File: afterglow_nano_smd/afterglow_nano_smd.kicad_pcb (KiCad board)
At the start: 2 copper layers, 113.7 x 80 mm, 112 parts, among them J1 J137_IN_C, J2 J133_IN_R, J3 Conn_Power, J4 J133_OUT_R, J5 J137_OUT_C, J6 J134_OUT_R, J7 J138_OUT_C, J8 J135_OUT_R, J9 136_OUT_C, Q1 IRF5305, Q10 IRL2905, Q11 IRL2905, Q12 IRL2905, Q13 IRL2905, Q14 IRL2905, Q15 IRL2905, Q16 IRL2905, Q2 IRF5305, Q3 IRF5305, Q4 IRF5305, Q5 IRF5305, Q6 IRF5305, Q7 IRF5305, Q8 IRF5305, Q9 IRL2905, SW1 CFG, U1 74LS165, U2 74LS165, U3 5V_Regulator, U4 arduino_nano, U5 74HC595, U6 74HC595, U7 ULN2803A

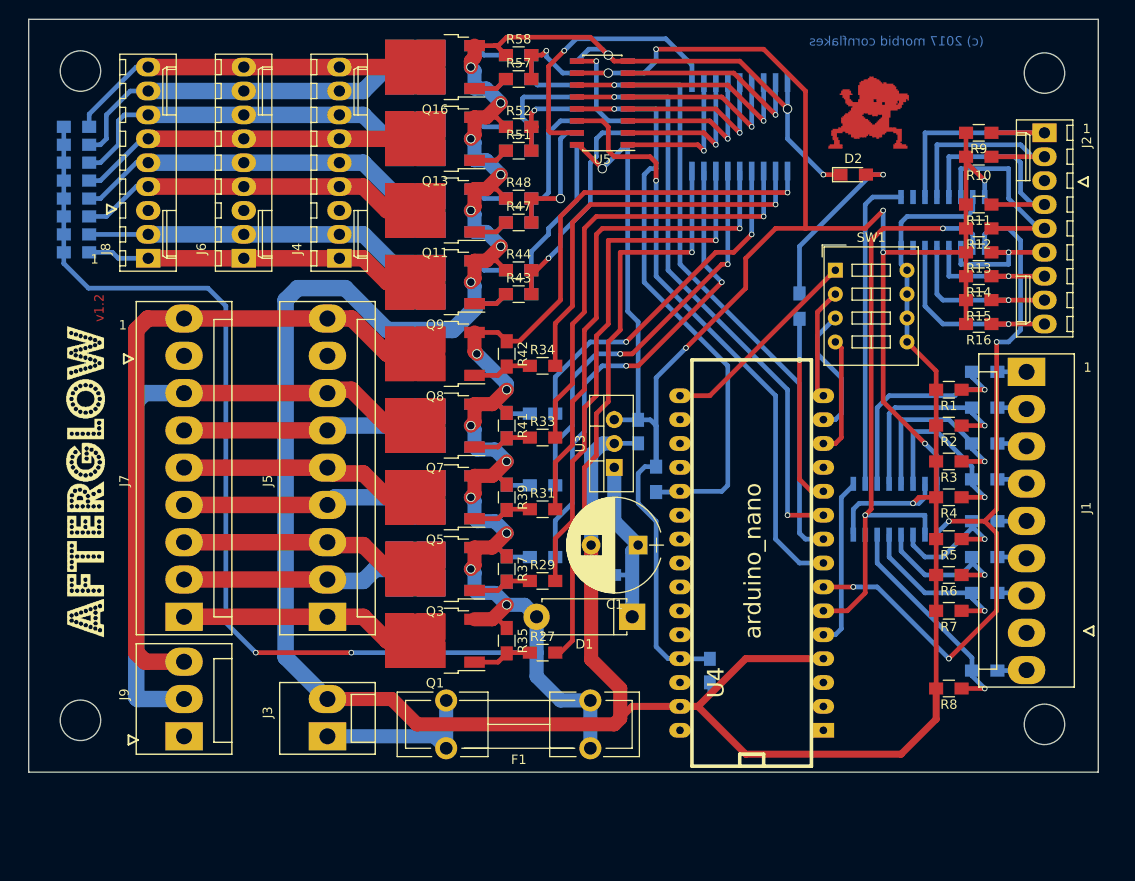
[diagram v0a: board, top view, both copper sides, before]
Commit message: v1.3 PCB progress
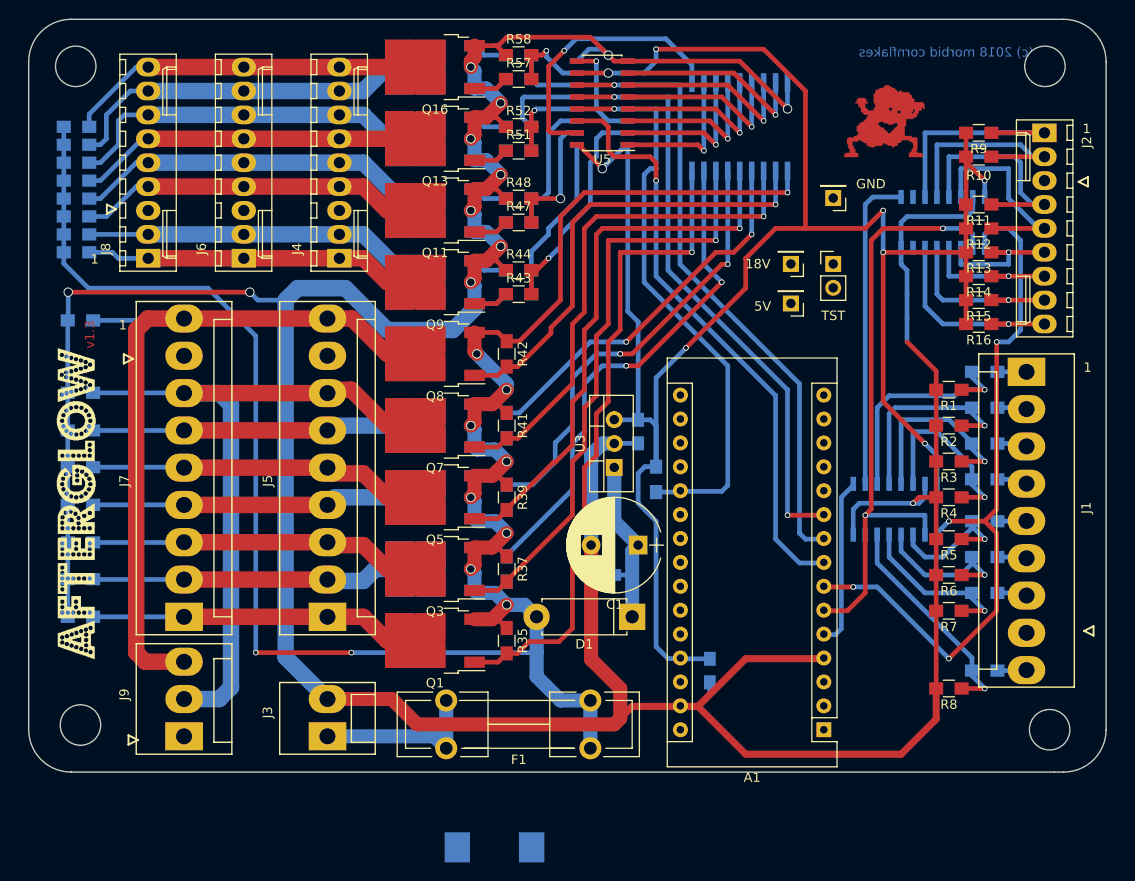
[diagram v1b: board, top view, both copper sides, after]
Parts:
- removed the ? at (132.9, 55.7)
- removed the ? at (30.5, 55.5)
- removed the ? at (30.5, 124.5)
- removed the ? at (132.9, 124.9)
- removed D2: LED, LEDs:LED_0805_HandSoldering
- removed SW1: CFG, Buttons_Switches_THT:SW_DIP_x4_W7.62mm_Slide
- removed U4: arduino_nano, arduino_nano:arduino_mini
- added 18V: TestPoint, Pin_Headers:Pin_Header_Straight_1x01_Pitch2.54mm, F.Cu at (106.0, 76.0)
- added 5V: TestPoint, Pin_Headers:Pin_Header_Straight_1x01_Pitch2.54mm, F.Cu at (106.0, 80.2)
- added ?: MountingHole_4.3mm_M4_ISO14580, Mounting_Holes:MountingHole_4.3mm_M4_ISO14580, F.Cu at (133.5, 125.5)
- added ?: MountingHole_4.3mm_M4_ISO14580, Mounting_Holes:MountingHole_4.3mm_M4_ISO14580, F.Cu at (133.0, 55.0)
- added ?: MountingHole_4.3mm_M4_ISO14580, Mounting_Holes:MountingHole_4.3mm_M4_ISO14580, F.Cu at (30.5, 125.0)
- added ?: MountingHole_4.3mm_M4_ISO14580, Mounting_Holes:MountingHole_4.3mm_M4_ISO14580, F.Cu at (30.0, 55.0)
- added A1: Arduino_Nano_v3.x, Modules:Arduino_Nano, F.Cu at (109.5, 125.5)
- added GND: TestPoint, Pin_Headers:Pin_Header_Straight_1x01_Pitch2.54mm, F.Cu at (110.5, 69.0)
- added TST: Jumper, Pin_Headers:Pin_Header_Straight_1x02_Pitch2.54mm, F.Cu at (110.5, 76.0)
- J1, J5, J7: footprint afterglow:Molex_KK-41791-9_9x3.96mm_Straight -> Connectors_Molex:Molex_KK-41791-9_9x3.96mm_Straight
- R1, R2, R3, R4, R5, R6, R7, R8: value 390 -> 330
- R26: value 220 -> 0.22; footprint Resistors_SMD:R_0805_HandSoldering -> Resistors_SMD:R_2512_HandSoldering
- R27, R29, R31, R33, R34: value 560 -> 10k; moved to B.Cu
- R28, R30, R32: value 560 -> 10k
- moved R26 66.0 mm to (74.5, 138.0), turned to 0 degrees
- moved R34 49.3 mm to (30.5, 82.0)
- moved R33 49.3 mm to (30.5, 89.7)
- moved R31 49.3 mm to (30.5, 97.6)
- moved R29 49.3 mm to (30.5, 105.6)
- moved R27 49.3 mm to (30.5, 113.5)
- moved R28 49.2 mm to (30.5, 109.5)
- moved R30 49.2 mm to (30.5, 101.6)
- moved R32 49.1 mm to (30.5, 93.7)
- moved afterglow 2.54 mm to (28.0, 118.0)
- moved FLAKIE 1.89 mm to (111.5, 57.0)
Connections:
- net VCC renamed /5V
- J1 pad 8: (no net) -> Net-(J1-Pad8)
- J2 pad 3: (no net) -> Net-(J2-Pad3)
- J4 pad 3: (no net) -> Net-(J4-Pad3)
- J5 pad 8: (no net) -> Net-(J5-Pad8)
- J6 pad 3: (no net) -> Net-(J6-Pad3)
- J7 pad 8: (no net) -> Net-(J7-Pad8)
- J8 pad 3: (no net) -> Net-(J8-Pad3)
- J9 pad 1: (no net) -> Net-(J9-Pad1)
- Q1 pad 1: Net-(Q1-Pad1) -> /CO1
- Q10 pad 3: GND -> /ROW_GND
- Q11 pad 3: GND -> /ROW_GND
- Q12 pad 3: GND -> /ROW_GND
- Q13 pad 3: GND -> /ROW_GND
- Q14 pad 3: GND -> /ROW_GND
- Q15 pad 3: GND -> /ROW_GND
- Q16 pad 3: GND -> /ROW_GND
- Q2 pad 1: Net-(Q2-Pad1) -> /CO2
- Q3 pad 1: Net-(Q3-Pad1) -> /CO3
- Q4 pad 1: Net-(Q4-Pad1) -> /CO4
- Q5 pad 1: Net-(Q5-Pad1) -> /CO5
- Q6 pad 1: Net-(Q6-Pad1) -> /CO6
- Q7 pad 1: Net-(Q7-Pad1) -> /CO7
- Q8 pad 1: Net-(Q8-Pad1) -> /CO8
- Q9 pad 3: GND -> /ROW_GND
- R26 pad 1: Net-(D2-Pad2) -> GND
- R26 pad 2: Net-(R26-Pad2) -> /ROW_GND
- R27 pad 1: Net-(Q1-Pad1) -> GND
- R27 pad 2: /CO1 -> /J137_CO1
- R28 pad 1: Net-(Q2-Pad1) -> GND
- R28 pad 2: /CO2 -> /J137_CO2
- R29 pad 1: Net-(Q3-Pad1) -> GND
- R29 pad 2: /CO3 -> /J137_CO3
- R30 pad 1: Net-(Q4-Pad1) -> GND
- R30 pad 2: /CO4 -> /J137_CO4
- R31 pad 1: Net-(Q5-Pad1) -> GND
- R31 pad 2: /CO5 -> /J137_CO5
- R32 pad 1: Net-(Q6-Pad1) -> GND
- R32 pad 2: /CO6 -> /J137_CO6
- R33 pad 1: Net-(Q7-Pad1) -> GND
- R33 pad 2: /CO7 -> /J137_CO7
- R34 pad 1: Net-(Q8-Pad1) -> GND
- R34 pad 2: /CO8 -> /J137_CO8
- R35 pad 2: Net-(Q1-Pad1) -> /CO1
- R36 pad 2: Net-(Q2-Pad1) -> /CO2
- R37 pad 2: Net-(Q3-Pad1) -> /CO3
- R38 pad 2: Net-(Q4-Pad1) -> /CO4
- R39 pad 2: Net-(Q5-Pad1) -> /CO5
- R40 pad 2: Net-(Q6-Pad1) -> /CO6
- R41 pad 2: Net-(Q7-Pad1) -> /CO7
- R42 pad 2: Net-(Q8-Pad1) -> /CO8
- R44 pad 1: GND -> /ROW_GND
- R46 pad 1: GND -> /ROW_GND
- R48 pad 1: GND -> /ROW_GND
- R50 pad 1: GND -> /ROW_GND
- R52 pad 1: GND -> /ROW_GND
- R54 pad 1: GND -> /ROW_GND
- R56 pad 1: GND -> /ROW_GND
- R58 pad 1: GND -> /ROW_GND
- U1 pad 7: (no net) -> Net-(U1-Pad7)
- U2 pad 10: (no net) -> Net-(U2-Pad10)
- U2 pad 7: (no net) -> Net-(U2-Pad7)
- U6 pad 9: (no net) -> Net-(U6-Pad9)
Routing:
- net GND: track 399.7 -> 447.3 mm, vias 11 -> 12
- net Net-(SW1-Pad1): track 22.0 -> 0.00 mm
- net Net-(R26-Pad2): track 20.1 -> 0.00 mm, vias 1 -> 0
- net Net-(D2-Pad2): track 18.9 -> 0.00 mm, vias 1 -> 0
- net Net-(SW1-Pad3): track 14.2 -> 0.00 mm
- net Net-(SW1-Pad4): track 12.6 -> 0.00 mm
- net Net-(SW1-Pad2): track 11.8 -> 0.00 mm
- net /J137_CO1: track 25.6 -> 35.6 mm
- net /J137_CO8: track 71.5 -> 81.2 mm
- net /J137_CO5: track 25.9 -> 35.6 mm
- net /J137_CO2: track 25.2 -> 34.8 mm
- net /J137_CO3: track 25.7 -> 35.4 mm
- net /J137_CO4: track 24.9 -> 34.6 mm
- net /J137_CO6: track 24.8 -> 34.4 mm
- net /J137_CO7: track 68.3 -> 77.0 mm
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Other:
- board size 113.7 x 80 mm -> 114.5 x 80 mm
- board text added: "(c) 2018 morbid cornflakes"
- board text added: "v1.3"

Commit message: v1.3 progressing
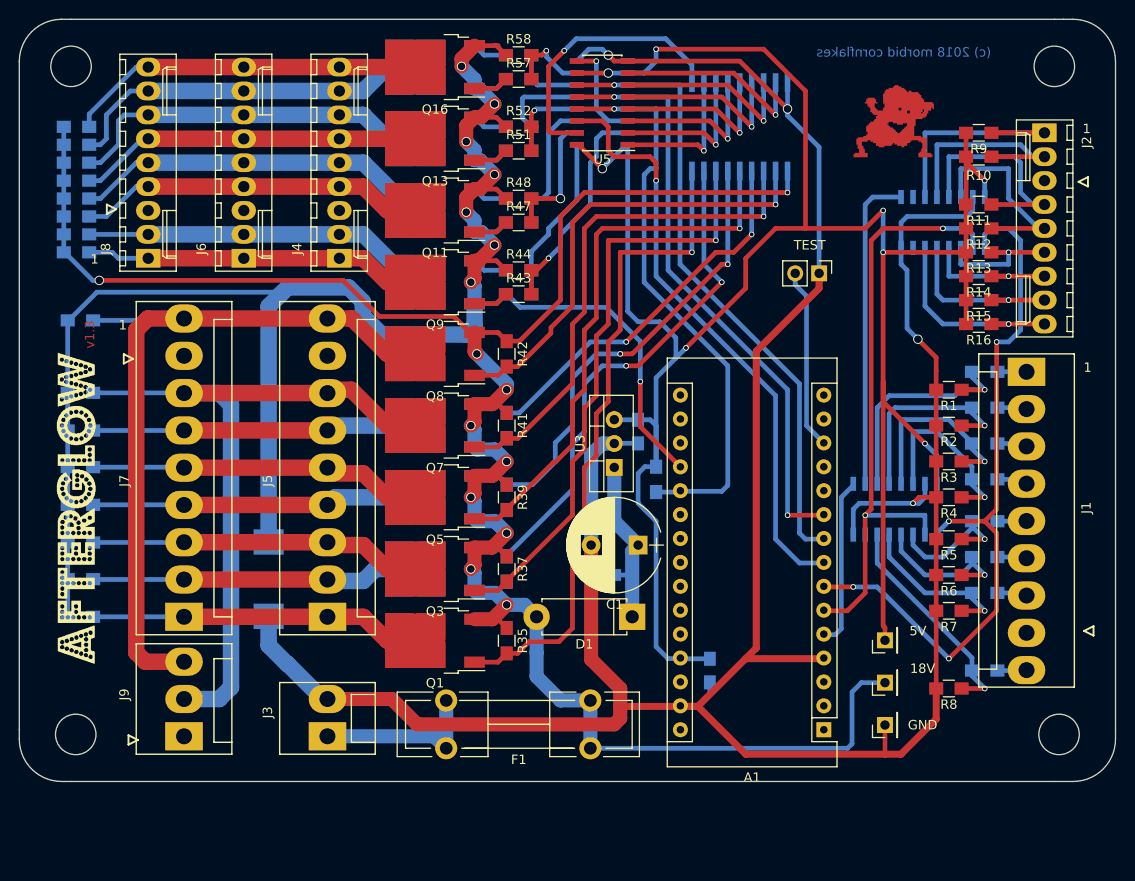
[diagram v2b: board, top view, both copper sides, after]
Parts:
- removed the ? at (133.5, 125.5)
- removed the ? at (133.0, 55.0)
- removed the ? at (30.5, 125.0)
- removed the ? at (30.0, 55.0)
- removed TST: Jumper, Pin_Headers:Pin_Header_Straight_1x02_Pitch2.54mm
- added ?: MountingHole_4.3mm_M4_ISO14580, Mounting_Holes:MountingHole_4.3mm_M4_ISO14580, F.Cu at (29.5, 55.0)
- added ?: MountingHole_4.3mm_M4_ISO14580, Mounting_Holes:MountingHole_4.3mm_M4_ISO14580, F.Cu at (30.0, 126.0)
- added ?: MountingHole_4.3mm_M4_ISO14580, Mounting_Holes:MountingHole_4.3mm_M4_ISO14580, F.Cu at (134.5, 126.0)
- added ?: MountingHole_4.3mm_M4_ISO14580, Mounting_Holes:MountingHole_4.3mm_M4_ISO14580, F.Cu at (134.0, 55.0)
- added TEST: Jumper, Pin_Headers:Pin_Header_Straight_1x02_Pitch2.54mm, F.Cu at (109.0, 77.0)
- moved GND 56.3 mm to (116.0, 125.0), turned to 90 degrees
- moved 18V 45.6 mm to (116.0, 120.5), turned to 90 degrees
- moved R26 37.3 mm to (50.5, 109.5), turned to 90 degrees
- moved 5V 37.2 mm to (116.0, 116.0), turned to 90 degrees
- moved FLAKIE 1.00 mm to (112.5, 57.0)
- moved afterglow 0.50 mm to (28.0, 118.5)
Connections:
- A1 pad 19: /ROW_GND -> /SUP_GND
- Q10 pad 3: /ROW_GND -> /SUP_GND
- Q11 pad 3: /ROW_GND -> /SUP_GND
- Q12 pad 3: /ROW_GND -> /SUP_GND
- Q13 pad 3: /ROW_GND -> /SUP_GND
- Q14 pad 3: /ROW_GND -> /SUP_GND
- Q15 pad 3: /ROW_GND -> /SUP_GND
- Q16 pad 3: /ROW_GND -> /SUP_GND
- Q9 pad 3: /ROW_GND -> /SUP_GND
- R26 pad 2: /ROW_GND -> /SUP_GND
- R27 pad 1: GND -> /SUP_GND
- R28 pad 1: GND -> /SUP_GND
- R29 pad 1: GND -> /SUP_GND
- R30 pad 1: GND -> /SUP_GND
- R31 pad 1: GND -> /SUP_GND
- R32 pad 1: GND -> /SUP_GND
- R33 pad 1: GND -> /SUP_GND
- R34 pad 1: GND -> /SUP_GND
- R44 pad 1: /ROW_GND -> /SUP_GND
- R46 pad 1: /ROW_GND -> /SUP_GND
- R48 pad 1: /ROW_GND -> /SUP_GND
- R50 pad 1: /ROW_GND -> /SUP_GND
- R52 pad 1: /ROW_GND -> /SUP_GND
- R54 pad 1: /ROW_GND -> /SUP_GND
- R56 pad 1: /ROW_GND -> /SUP_GND
- R58 pad 1: /ROW_GND -> /SUP_GND
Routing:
- net /SUP_GND: track 0.00 -> 209.9 mm, vias 0 -> 8
- net GND: track 447.3 -> 315.2 mm, vias 12 -> 4
- net /5V: track 225.6 -> 249.6 mm
- net Net-(A1-Pad13): track 0.00 -> 19.3 mm
- net /18V: track 248.4 -> 244.7 mm, vias 11 -> 10
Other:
- board size 114.5 x 80 mm -> 116.5 x 81 mm
